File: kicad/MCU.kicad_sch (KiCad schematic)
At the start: 78 parts, among them J3 USART, J4 FAN, J5 USB_A, J6 Display, Q7 2N7002NXAK, Q8 2N7002K, Q9 2N7002K, SW1 ENC0 (Voltage), SW2 ENC1 (Current), SW3 BOOT, SW4 RST, U6 USBLC6-2SC6, U7 MCP9700A, U8 STM32F373C8Tx, Y1 Crystal

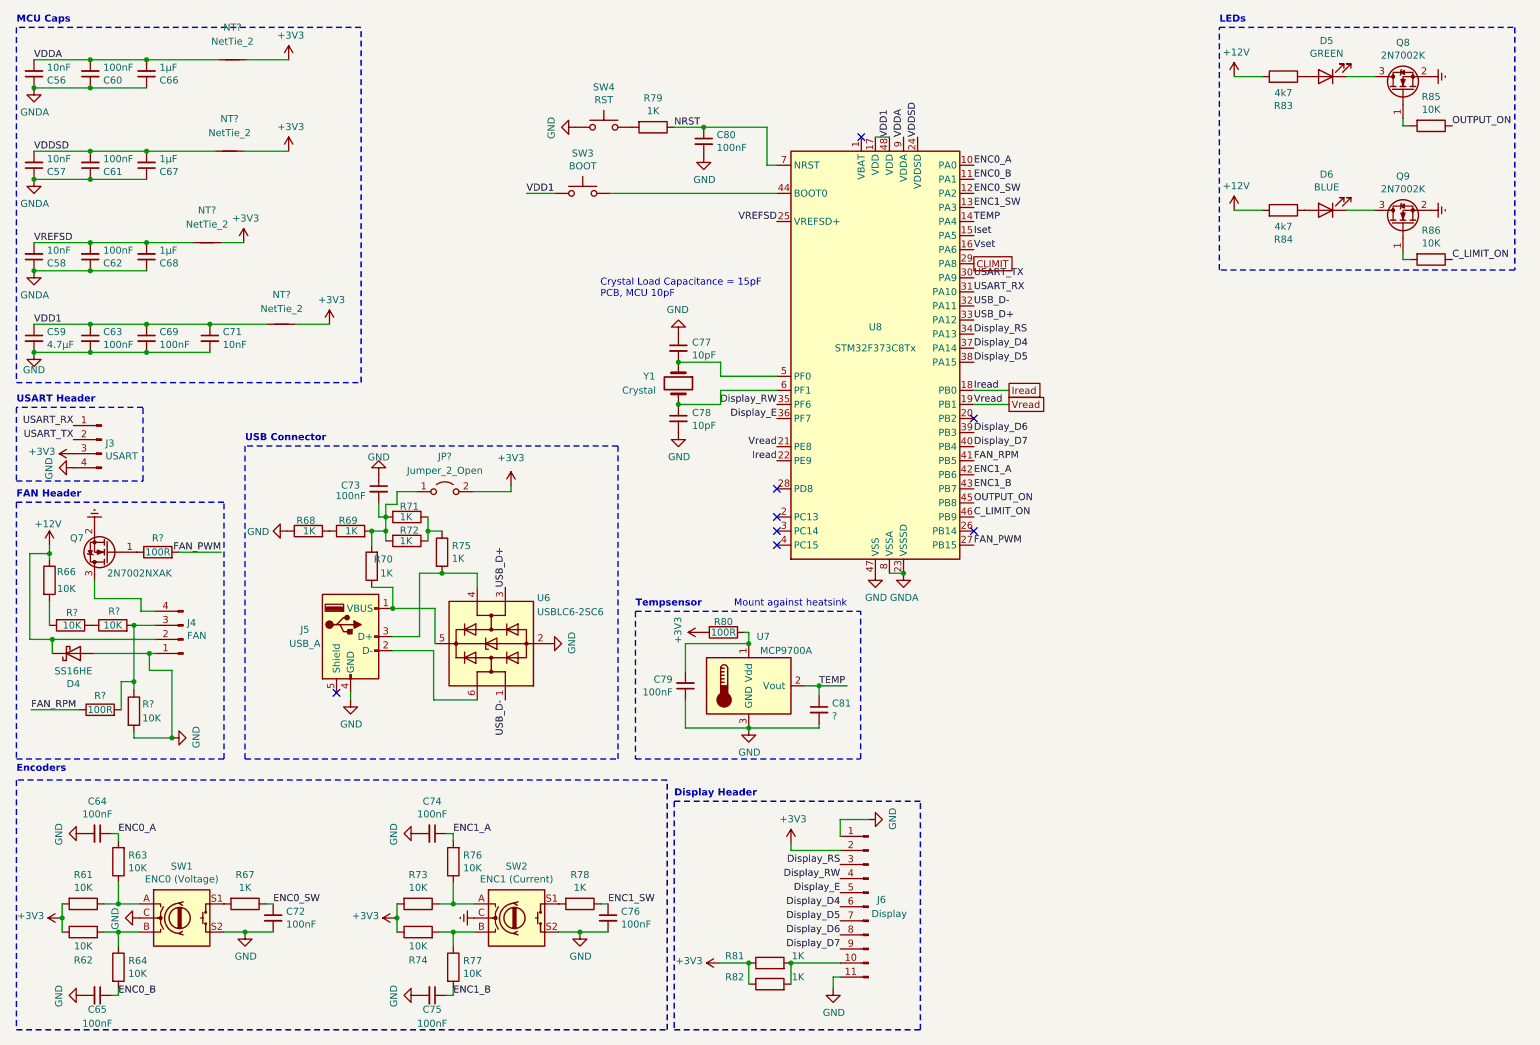
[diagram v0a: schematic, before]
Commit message: Fixed a bunch of alignment
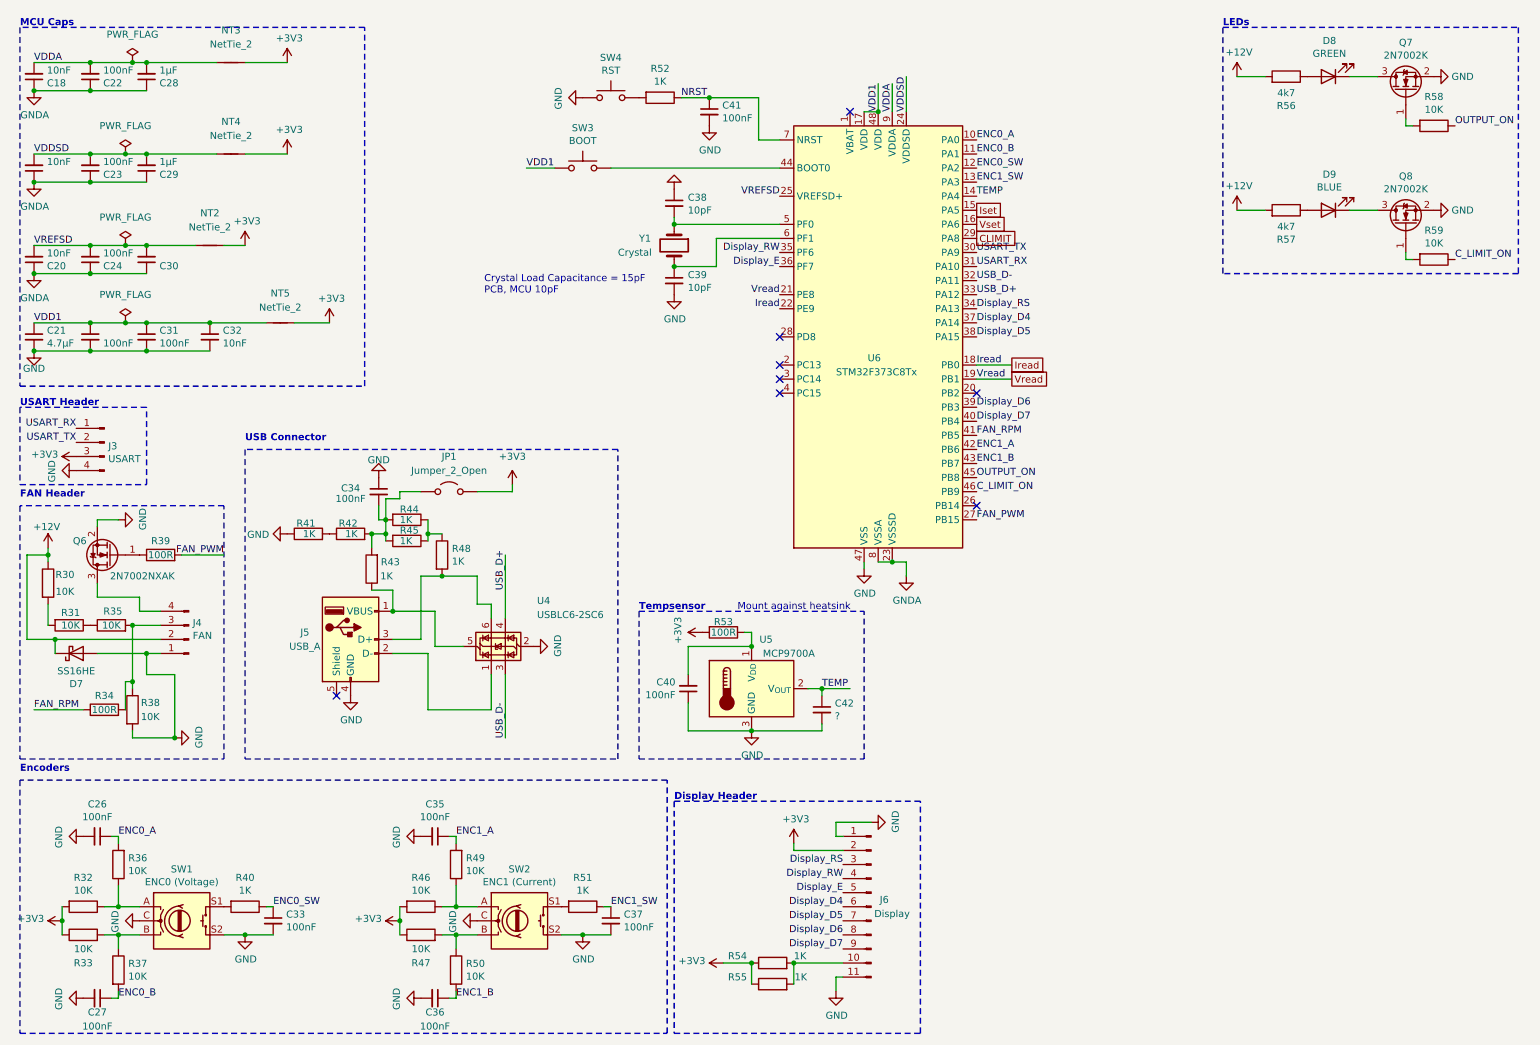
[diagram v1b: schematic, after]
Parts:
- removed U8: STM32F373C8Tx, Package_QFP:LQFP-48_7x7mm_P0.5mm, symbol MCU_ST_STM32F3:STM32F373C8Tx
- added U6: STM32F373C8Tx, Package_QFP:LQFP-48_7x7mm_P0.5mm, symbol MCU_ST_STM32F3:STM32F373C8Tx
- J3, J4: symbol Connector:Conn_01x04_Male -> Connector:Conn_01x04_Pin
- J6: symbol Connector:Conn_01x11_Male -> Connector:Conn_01x11_Pin
- U5: renamed from U7; footprint Package_TO_SOT_THT:TO-92_Inline -> Package_TO_SOT_SMD:SOT-23; symbol Sensor_Temperature:MCP9700AT-ETT -> Sensor_Temperature:MCP9700Ax-ETT
- gave numbers to parts that had none: 10
- renumbered C56 to C18, C57 to C19, C58 to C20, C59 to C21, C60 to C22, C61 to C23, C62 to C24, C63 to C25, C64 to C26, C65 to C27, C66 to C28, C67 to C29, C68 to C30, C69 to C31, C71 to C32, C72 to C33, C73 to C34, C74 to C35, C75 to C36, C76 to C37, C77 to C38, C78 to C39, C79 to C40, C80 to C41, C81 to C42, D4 to D7, D5 to D8, D6 to D9, Q7 to Q6, Q8 to Q7, Q9 to Q8, R66 to R30, R61 to R32, R62 to R33, R63 to R36, R64 to R37, R67 to R40, R68 to R41, R69 to R42, R70 to R43, R71 to R44, R72 to R45, R73 to R46, R74 to R47, R75 to R48, R76 to R49, R77 to R50, R78 to R51, R79 to R52, R80 to R53, R81 to R54, R82 to R55, R83 to R56, R84 to R57, R85 to R58, R86 to R59, U6 to U4
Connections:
- net GNDREF is gone; now on net GND: Q6.2 (S), Q7.2 (S), Q8.2 (S), SW2.C
- net CLIMIT: now also U6.29 (PA8)
- net C_LIMIT_ON: now also U6.46 (PB9)
- net Display_D4: now also U6.37 (PA14)
- net Display_D5: now also U6.38 (PA15)
- net Display_D6: now also U6.39 (PB3)
- net Display_D7: now also U6.40 (PB4)
- net Display_E: now also U6.36 (PF7)
- net Display_RS: now also U6.34 (PA13)
- net Display_RW: now also U6.35 (PF6)
- net ENC0_A: now also U6.10 (PA0)
- net ENC0_B: now also U6.11 (PA1)
- net ENC0_SW: now also U6.12 (PA2)
- net ENC1_A: now also U6.42 (PB6)
- net ENC1_B: now also U6.43 (PB7)
- net ENC1_SW: now also U6.13 (PA3)
- net FAN_PWM: now also U6.27 (PB15)
- net FAN_RPM: now also U6.41 (PB5)
- net GND: now also U6.47 (VSS)
- net GNDA: now also U6.23 (VSSSD), U6.8 (VSSA)
- net Iread: now also U6.18 (PB0), U6.22 (PE9)
- net Iset: now also U6.15 (PA5)
- net NRST: now also U6.7 (NRST)
- net OUTPUT_ON: now also U6.45 (PB8)
- net TEMP: now also U6.14 (PA4)
- net USART_RX: now also U6.31 (PA10)
- net USART_TX: now also U6.30 (PA9)
- net USB_D+: now also U4.4 (I/O2), U6.33 (PA12); no longer U4.3 (I/O2)
- net USB_D-: now also U4.3 (I/O2), U6.32 (PA11); no longer U4.1 (I/O1)
- net VDD1: now also U6.17 (VDD), U6.48 (VDD)
- net VDDA: now also U6.9 (VDDA)
- net VDDSD: now also U6.24 (VDDSD)
- net VREFSD: now also U6.25 (VREFSD+)
- net Vread: now also U6.19 (PB1), U6.21 (PE8)
- net Vset: now also U6.16 (PA6)
- net at J5.3 (D+), R48.2: now also U4.6 (I/O1); no longer U4.4 (I/O2)
- net at J5.2 (D-): now also U4.1 (I/O1); no longer U4.6 (I/O1)
- net at SW3.1: now also U6.44 (BOOT0)
- net at C38.2, Y1.1: now also U6.5 (PF0)
- net at C39.1, Y1.2: now also U6.6 (PF1)
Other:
- moved on the sheet: C18, C20, C22, C23, C24, C26, C27, C28, C29, C30, C33, C34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
